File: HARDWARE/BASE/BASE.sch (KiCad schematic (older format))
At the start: 0 parts

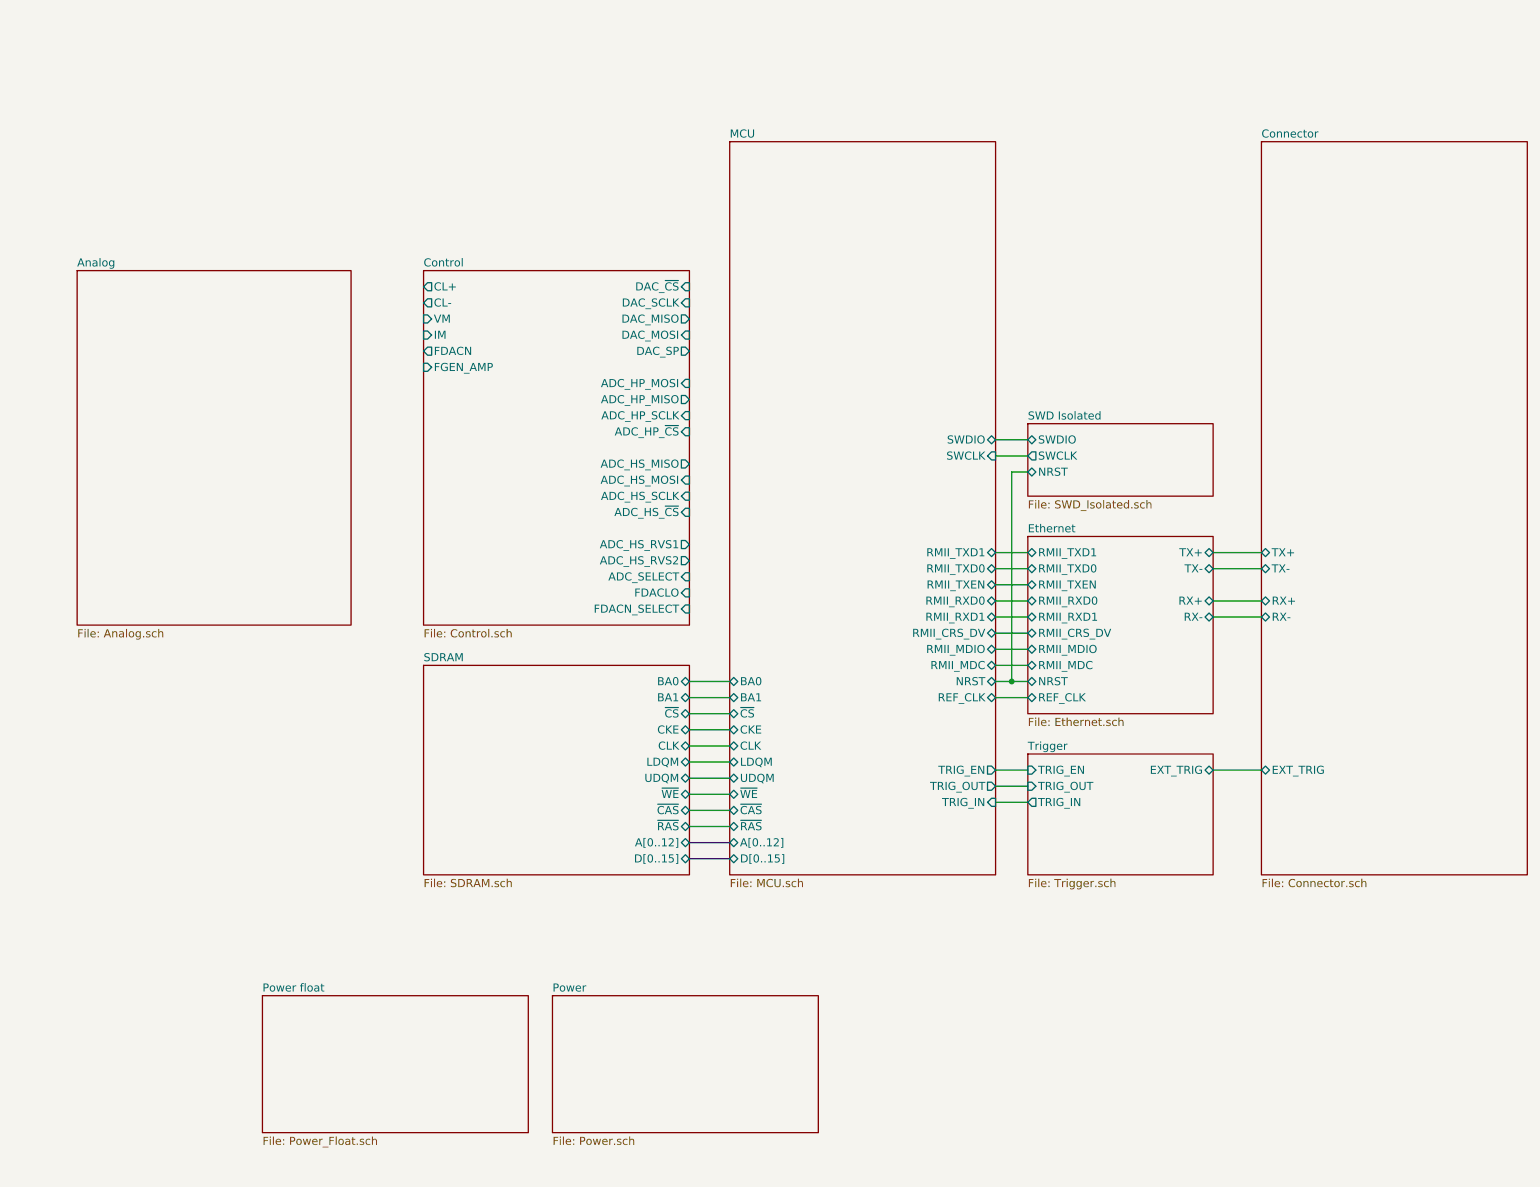
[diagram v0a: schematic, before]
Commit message: Schematic design.
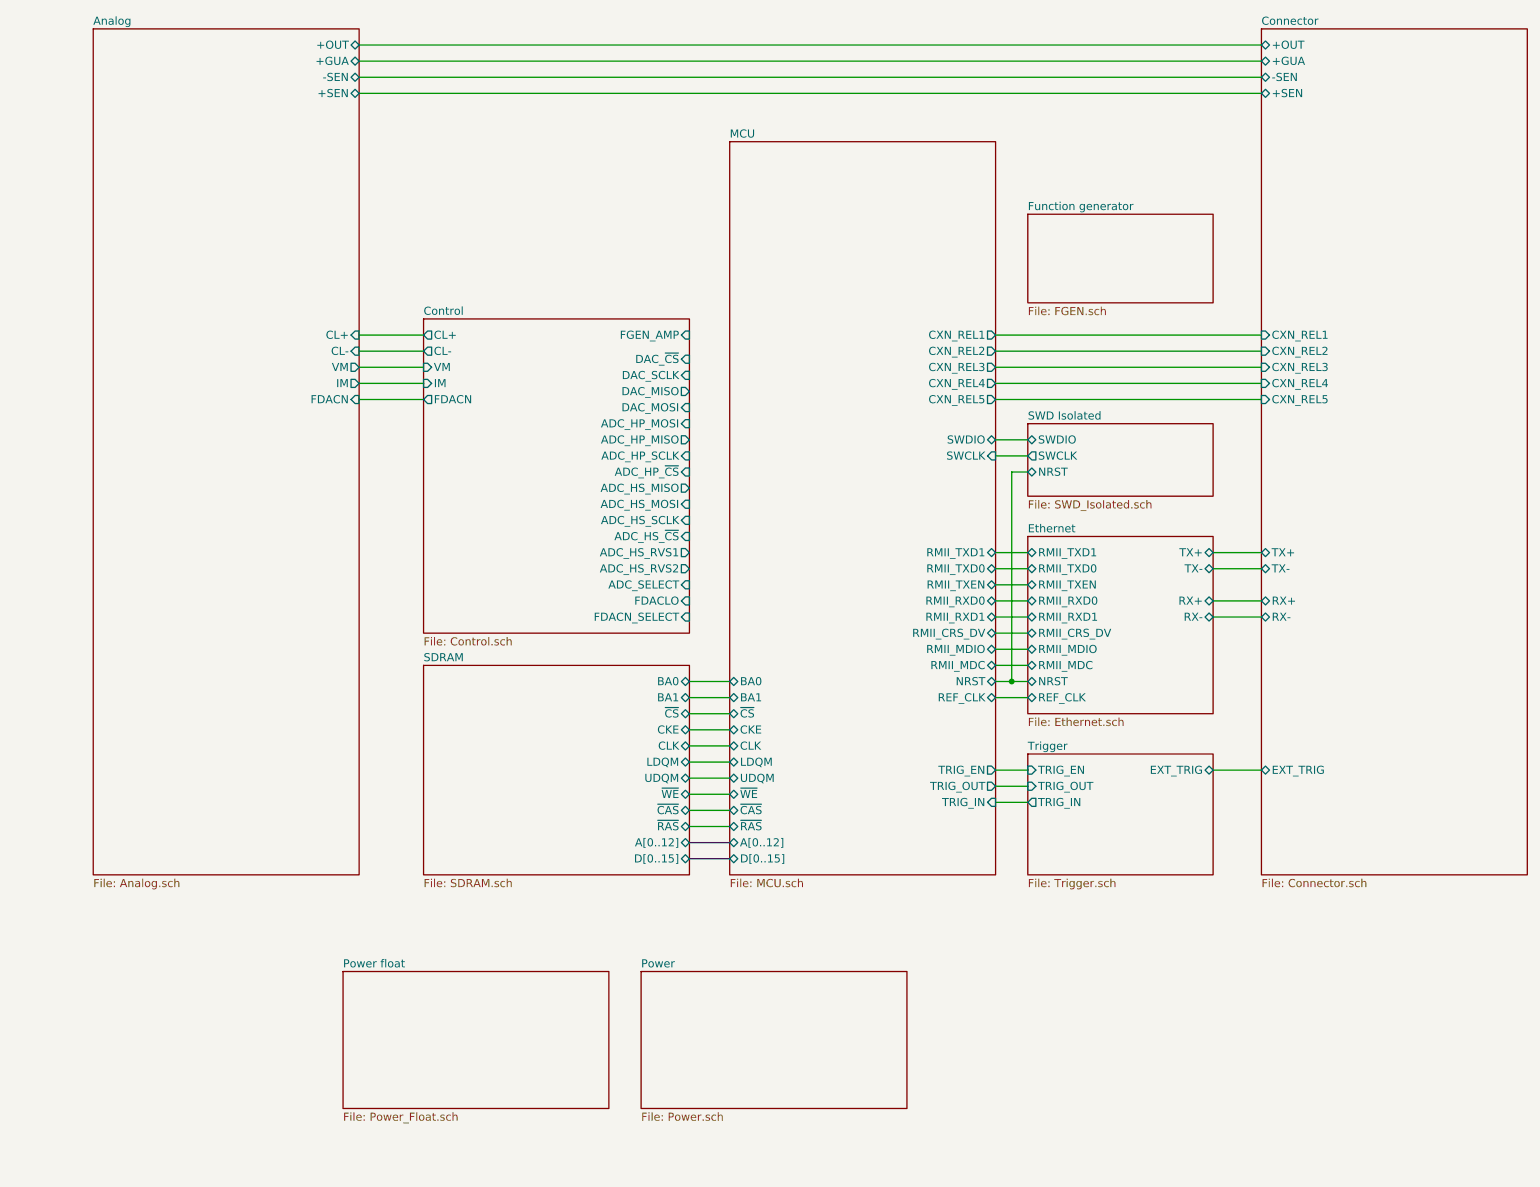
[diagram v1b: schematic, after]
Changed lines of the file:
@@
 $Descr A4 11693 8268
 encoding utf-8
-Sheet 1 11
+Sheet 1 12
 Title ""
 Date ""
@@
 F27 "SWDIO" B R 7250 3250 50
 F28 "SWCLK" I R 7250 3350 50
-$EndSheet
-$Sheet
-S 8900 1400 1650 4550
+F29 "CXN_REL5" O R 7250 3000 50
+F30 "CXN_REL4" O R 7250 2900 50
+F31 "CXN_REL3" O R 7250 2800 50
+F32 "CXN_REL2" O R 7250 2700 50
+F33 "CXN_REL1" O R 7250 2600 50
+$EndSheet
+$Sheet
+S 8900 700  1650 5250
 U 607E0822
 F0 "Connector" 50
@@
 F5 "RX+" B L 8900 4250 50
 F6 "EXT_TRIG" B L 8900 5300 50
+F7 "+OUT" B L 8900 800 50
+F8 "+GUA" B L 8900 900 50
+F9 "-SEN" B L 8900 1000 50
+F10 "+SEN" B L 8900 1100 50
+F11 "CXN_REL5" I L 8900 3000 50
+F12 "CXN_REL4" I L 8900 2900 50
+F13 "CXN_REL3" I L 8900 2800 50
+F14 "CXN_REL2" I L 8900 2700 50
+F15 "CXN_REL1" I L 8900 2600 50
 $EndSheet
 Wire Wire Line
@@
 	8900 3950 8600 3950
 $Sheet
-S 4500 6700 1650 850
+S 5050 6550 1650 850
 U 6051575A
 F0 "Power" 50
@@
 $EndSheet
 $Sheet
-S 2700 6700 1650 850
+S 3200 6550 1650 850
 U 6054E524
 F0 "Power float" 50
@@
 $EndSheet
 $Sheet
-S 3700 2200 1650 2200
+S 3700 2500 1650 1950
 U 608EADFA
 F0 "Control" 50
 F1 "Control.sch" 50
-F2 "DAC_~CS" I R 5350 2300 50
-F3 "DAC_SCLK" I R 5350 2400 50
-F4 "DAC_MISO" O R 5350 2500 50
-F5 "DAC_MOSI" I R 5350 2600 50
-F6 "DAC_SP" O R 5350 2700 50
-F7 "CL+" O L 3700 2300 50
-F8 "CL-" O L 3700 2400 50
-F9 "VM" I L 3700 2500 50
-F10 "IM" I L 3700 2600 50
-F11 "ADC_HP_MOSI" I R 5350 2900 50
-F12 "ADC_HP_MISO" O R 5350 3000 50
-F13 "ADC_HP_SCLK" I R 5350 3100 50
-F14 "ADC_HP_~CS" I R 5350 3200 50
-F15 "ADC_SELECT" I R 5350 4100 50
-F16 "ADC_HS_MOSI" I R 5350 3500 50
-F17 "ADC_HS_MISO" O R 5350 3400 50
-F18 "ADC_HS_SCLK" I R 5350 3600 50
-F19 "ADC_HS_~CS" I R 5350 3700 50
-F20 "ADC_HS_RVS1" O R 5350 3900 50
-F21 "ADC_HS_RVS2" O R 5350 4000 50
-F22 "FDACN_SELECT" I R 5350 4300 50
-F23 "FGEN_AMP" I L 3700 2800 50
-F24 "FDACLO" I R 5350 4200 50
-F25 "FDACN" O L 3700 2700 50
-$EndSheet
-$Sheet
-S 1550 2200 1700 2200
+F2 "DAC_~CS" I R 5350 2750 50
+F3 "DAC_SCLK" I R 5350 2850 50
+F4 "DAC_MISO" O R 5350 2950 50
+F5 "DAC_MOSI" I R 5350 3050 50
+F6 "CL+" O L 3700 2600 50
+F7 "CL-" O L 3700 2700 50
+F8 "VM" I L 3700 2800 50
+F9 "IM" I L 3700 2900 50
+F10 "ADC_HP_MOSI" I R 5350 3150 50
+F11 "ADC_HP_MISO" O R 5350 3250 50
+F12 "ADC_HP_SCLK" I R 5350 3350 50
+F13 "ADC_HP_~CS" I R 5350 3450 50
+F14 "ADC_SELECT" I R 5350 4150 50
+F15 "ADC_HS_MOSI" I R 5350 3650 50
+F16 "ADC_HS_MISO" O R 5350 3550 50
+F17 "ADC_HS_SCLK" I R 5350 3750 50
+F18 "ADC_HS_~CS" I R 5350 3850 50
+F19 "ADC_HS_RVS1" O R 5350 3950 50
+F20 "ADC_HS_RVS2" O R 5350 4050 50
+F21 "FDACN_SELECT" I R 5350 4350 50
+F22 "FGEN_AMP" I R 5350 2600 50
+F23 "FDACLO" I R 5350 4250 50
+F24 "FDACN" O L 3700 3000 50
+$EndSheet
+$Sheet
+S 1650 700  1650 5250
 U 60575ED4
 F0 "Analog" 50
 F1 "Analog.sch" 50
+F2 "CL+" I R 3300 2600 50
+F3 "CL-" I R 3300 2700 50
+F4 "FDACN" I R 3300 3000 50
+F5 "VM" O R 3300 2800 50
+F6 "IM" O R 3300 2900 50
+F7 "+OUT" B R 3300 800 50
+F8 "+GUA" B R 3300 900 50
+F9 "-SEN" B R 3300 1000 50
+F10 "+SEN" B R 3300 1100 50
 $EndSheet
 $Sheet
@@
 Wire Wire Line
 	7350 4750 7250 4750
+Wire Wire Line
+	3300 800  8900 800
+Wire Wire Line
+	3300 900  8900 900
+Wire Wire Line
+	3300 1000 8900 1000
+Wire Wire Line
+	3300 1100 8900 1100
+Wire Wire Line
+	7250 3000 8900 3000
+Wire Wire Line
+	7250 2900 8900 2900
+Wire Wire Line
+	8900 2800 7250 2800
+Wire Wire Line
+	7250 2700 8900 2700
+Wire Wire Line
+	8900 2600 7250 2600
+Wire Wire Line
+	3300 3000 3700 3000
+Wire Wire Line
+	3300 2900 3700 2900
+Wire Wire Line
+	3700 2800 3300 2800
+Wire Wire Line
+	3300 2700 3700 2700
+Wire Wire Line
+	3700 2600 3300 2600
+$Sheet
+S 7450 1850 1150 550
+U 627FE945
+F0 "Function generator" 50
+F1 "FGEN.sch" 50
+$EndSheet
 $EndSCHEMATC

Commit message: Schematic design
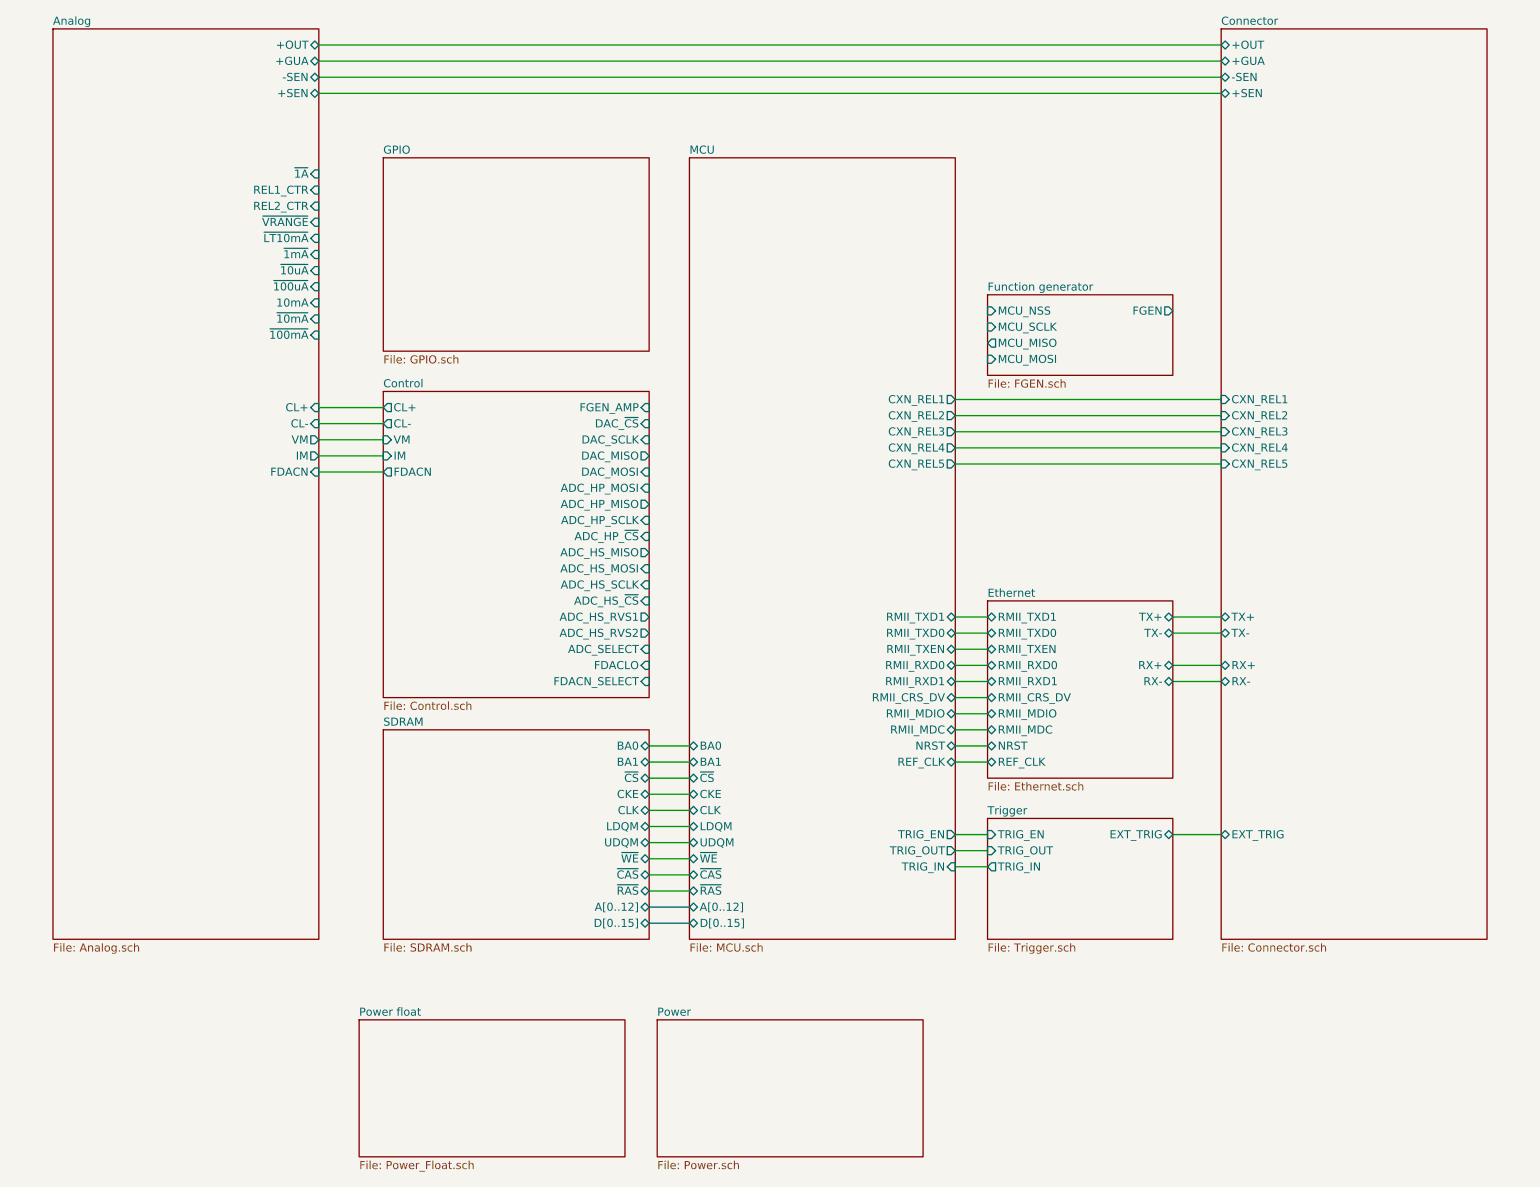
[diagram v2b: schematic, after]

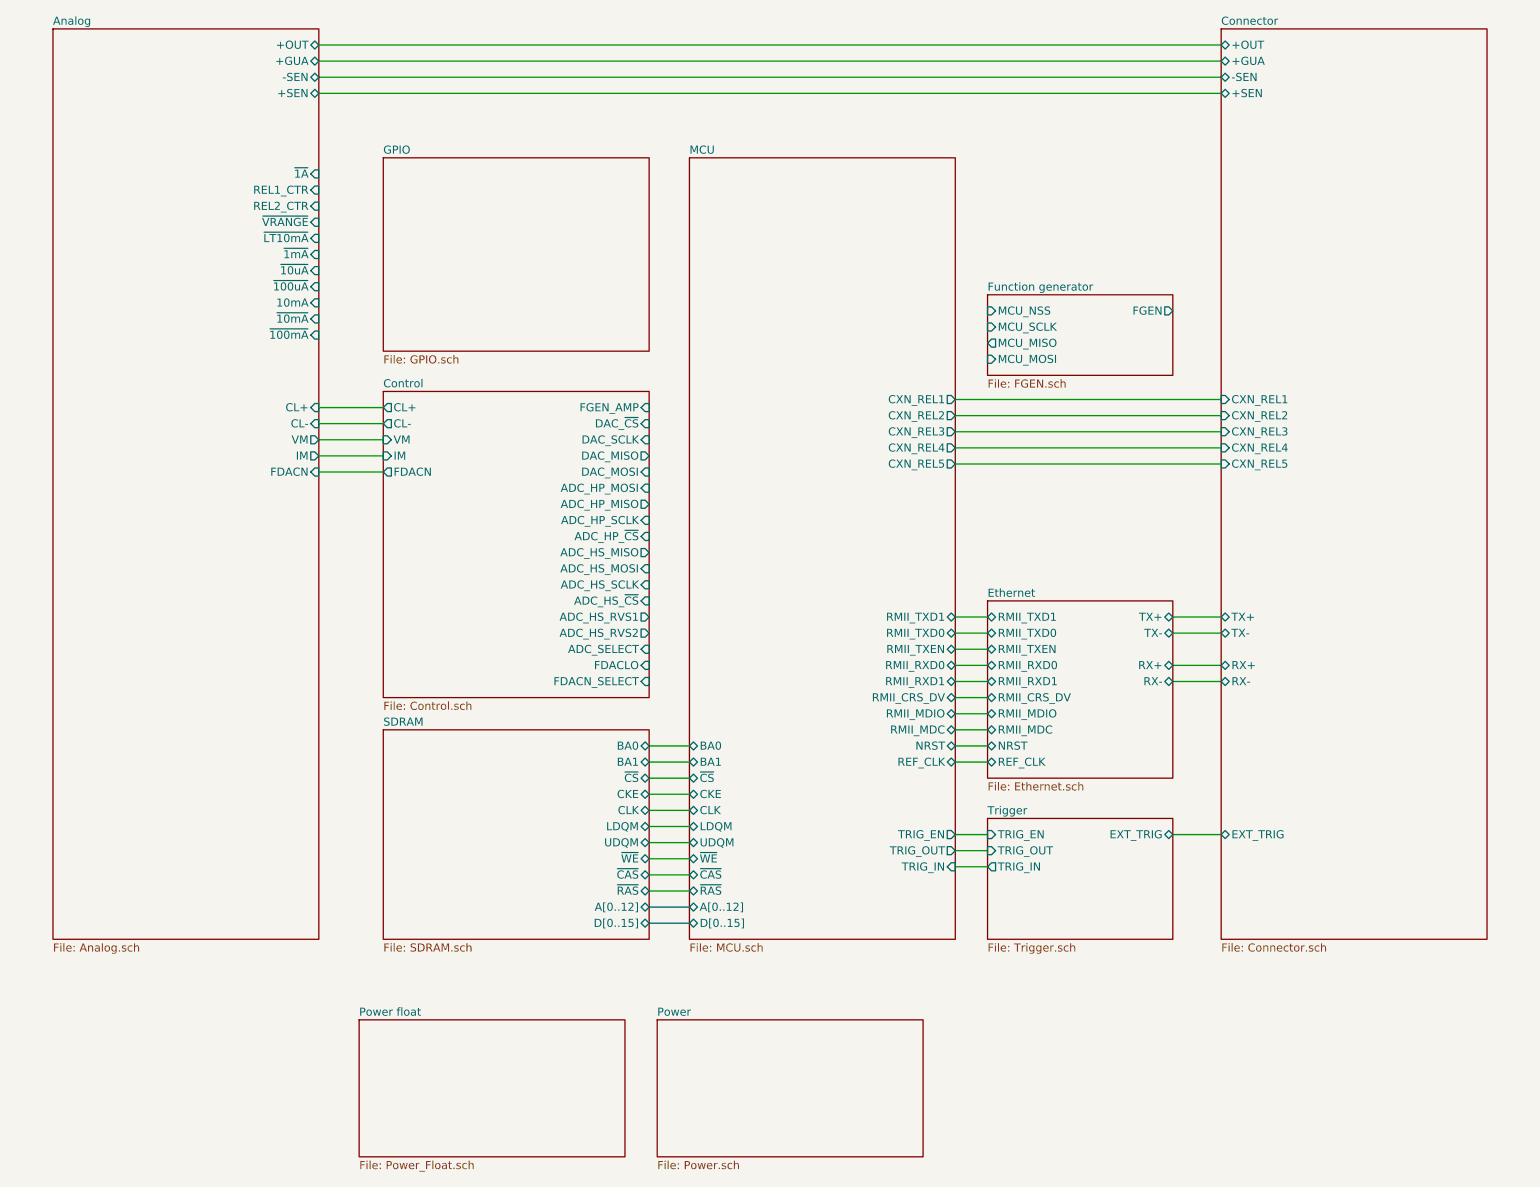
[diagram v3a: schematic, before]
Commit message: Design
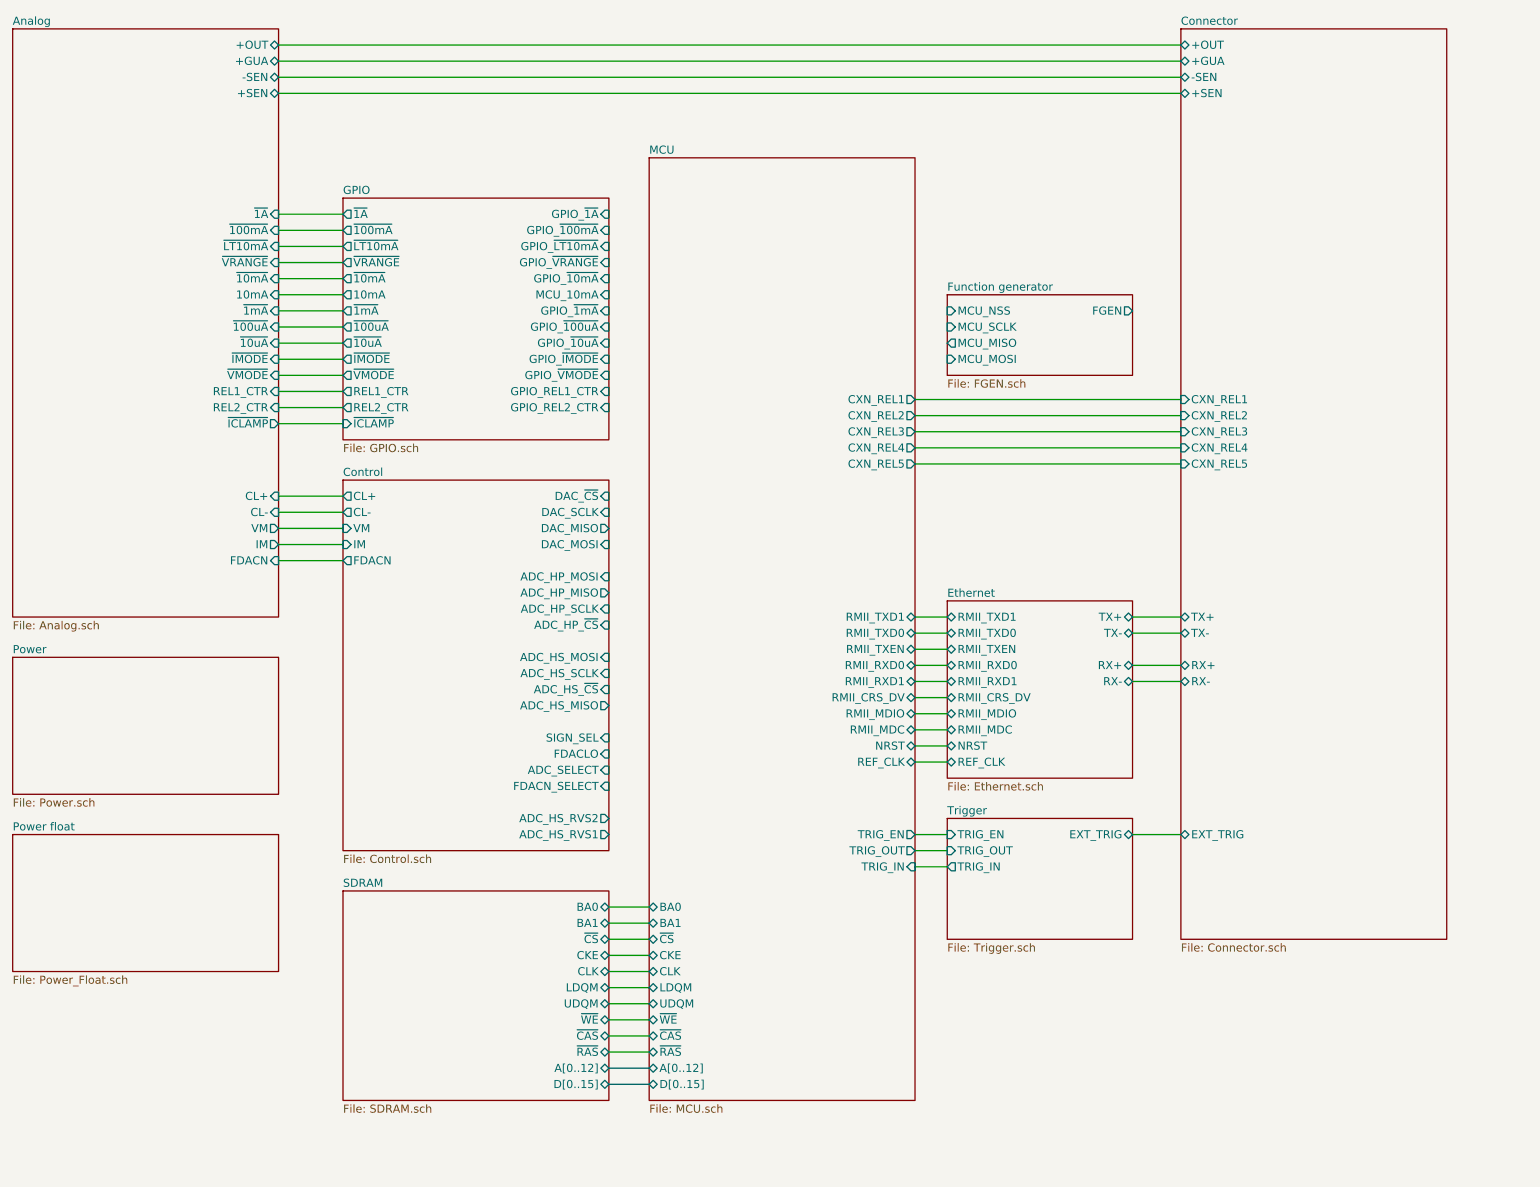
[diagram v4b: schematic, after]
